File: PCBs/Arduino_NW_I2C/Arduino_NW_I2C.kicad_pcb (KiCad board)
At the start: 2 copper layers, 68.6 x 53.3 mm, 22 parts, among them J1 PT_Conn_01x04, J10 PT_Conn_01x04, J11 PT_Conn_01x04, J12 PT_Conn_01x04, J13 PT_Conn_01x04, J14 Conn_01x02_Female, J2 PT_Conn_01x06, J3 PT_Conn_01x06, J4 PT_Conn_01x06, J5 PT_Conn_01x06, J6 Conn_01x08_Female, J7 Conn_01x08_Female, J8 Conn_01x08_Female, J9 PT_Conn_01x04, U1 PT_Ethernet_Shield, U2 MUX

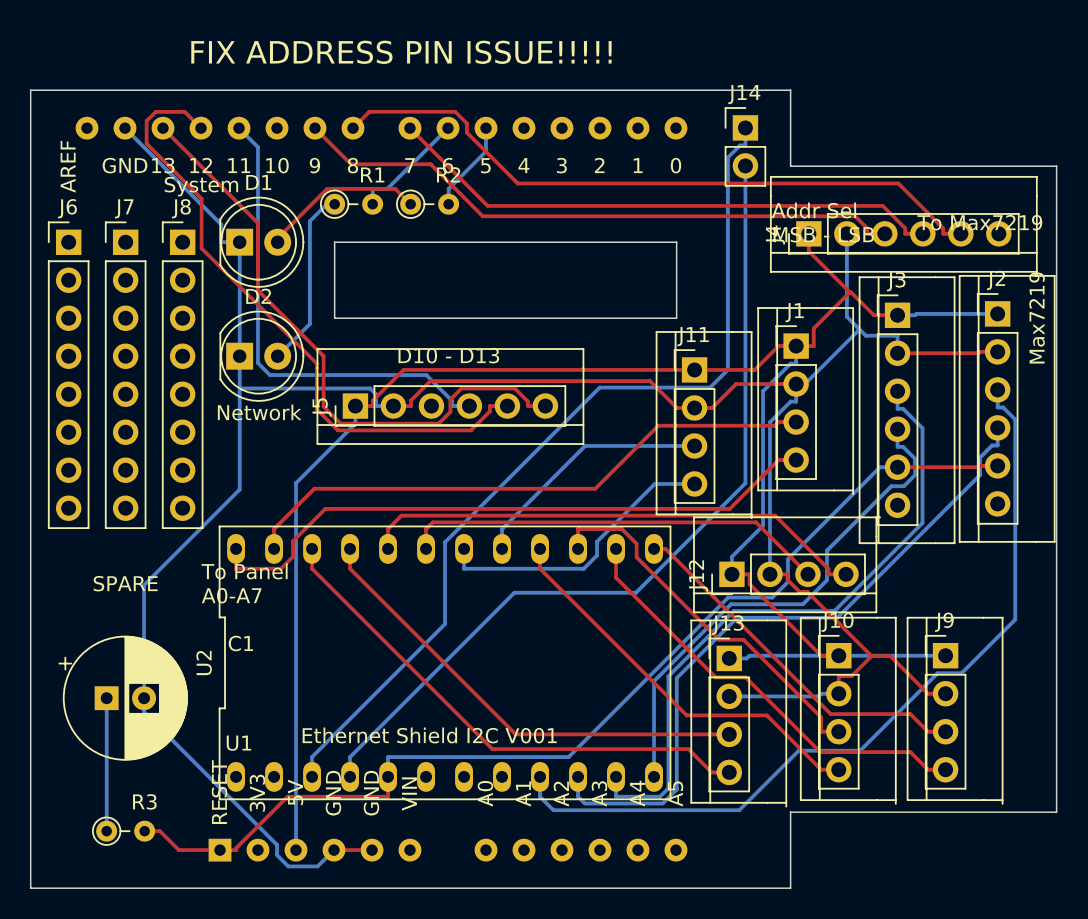
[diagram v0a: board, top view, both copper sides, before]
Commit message: PCB WORK
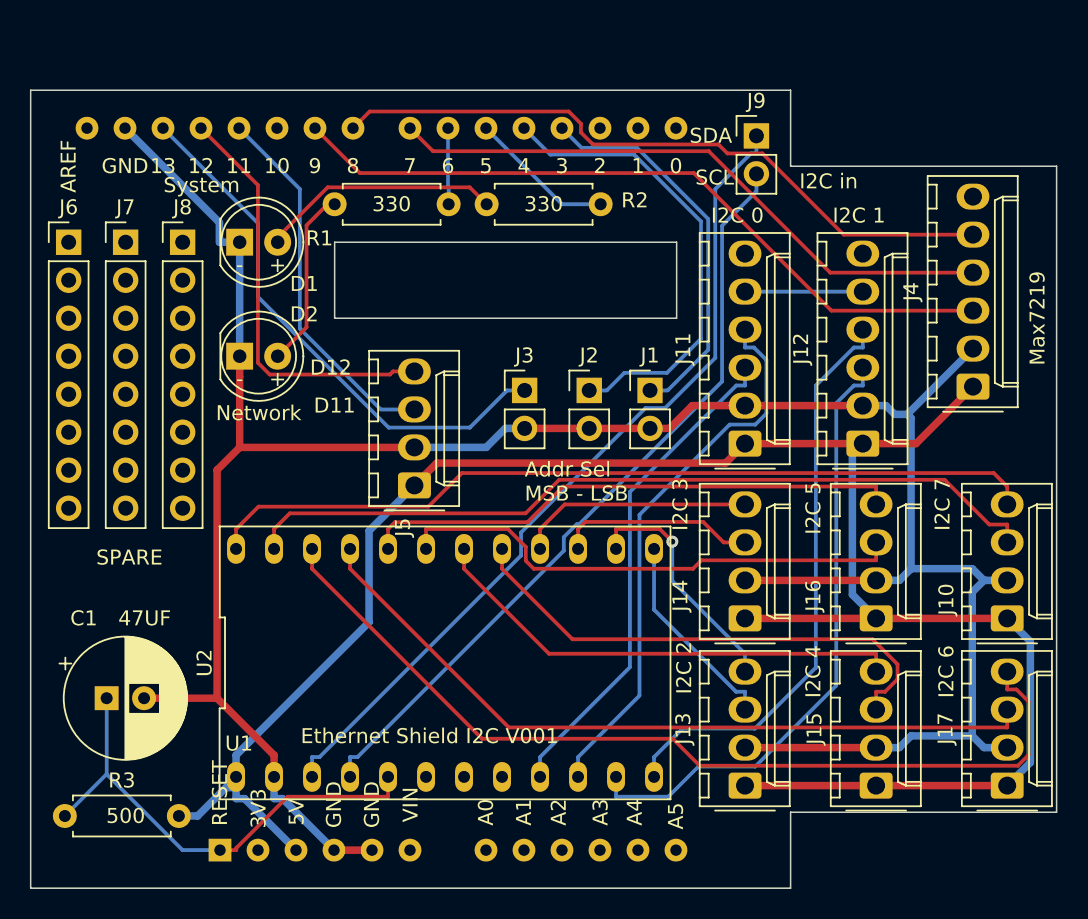
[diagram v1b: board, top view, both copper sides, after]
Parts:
- removed the J10 at (152.4, 101.0)
- added J1: A0, Connector_PinHeader_2.54mm:PinHeader_1x02_P2.54mm_Vertical, F.Cu at (139.8, 83.3)
- added J14: PT_Conn_01x04, PT_Library_v001:Molex_1x04_P2.54mm_Vertical, F.Cu at (146.2, 98.6)
- added J2: A1, Connector_PinHeader_2.54mm:PinHeader_1x02_P2.54mm_Vertical, F.Cu at (135.7, 83.3)
- added J3: A2, Connector_PinHeader_2.54mm:PinHeader_1x02_P2.54mm_Vertical, F.Cu at (131.4, 83.3)
- J10: renamed from J1; footprint PT_Library_v001:PT_PinHeader_1x04_P2.54mm_Vertical -> PT_Library_v001:Molex_1x04_P2.54mm_Vertical
- J11: renamed from J2; footprint PT_Library_v001:PT_PinHeader_1x06_P2.54mm_Vertical -> PT_Library_v001:Molex_1x06_P2.54mm_Vertical
- J12: renamed from J3; footprint PT_Library_v001:PT_PinHeader_1x06_P2.54mm_Vertical -> PT_Library_v001:Molex_1x06_P2.54mm_Vertical
- J13: renamed from J9; footprint PT_Library_v001:PT_PinHeader_1x04_P2.54mm_Vertical -> PT_Library_v001:Molex_1x04_P2.54mm_Vertical
- J15: renamed from J11; footprint PT_Library_v001:PT_PinHeader_1x04_P2.54mm_Vertical -> PT_Library_v001:Molex_1x04_P2.54mm_Vertical
- J16: renamed from J12; footprint PT_Library_v001:PT_PinHeader_1x04_P2.54mm_Vertical -> PT_Library_v001:Molex_1x04_P2.54mm_Vertical
- J17: renamed from J13; footprint PT_Library_v001:PT_PinHeader_1x04_P2.54mm_Vertical -> PT_Library_v001:Molex_1x04_P2.54mm_Vertical
- J4: footprint PT_Library_v001:PT_PinHeader_1x06_P2.54mm_Vertical -> PT_Library_v001:Molex_1x06_P2.54mm_Vertical
- J5: footprint PT_Library_v001:PT_PinHeader_1x06_P2.54mm_Vertical -> PT_Library_v001:Molex_1x04_P2.54mm_Vertical
- R1, R2, R3: footprint PT_Library_v001:PT_R_Axial_DIN0204_L3.6mm_D1.6mm_P2.54mm_Vertical -> PT_Library_v001:R_Axial_DIN0207_L6.3mm_D2.5mm_P7.62mm_Horizontal
- moved J15 30.3 mm to (154.9, 109.7), turned to 90 degrees
- moved J10 23.0 mm to (163.7, 98.6), turned to 90 degrees
- moved J17 20.4 mm to (163.7, 109.7), turned to 90 degrees
- moved J11 19.0 mm to (146.2, 86.9), turned to 90 degrees
- moved J13 16.0 mm to (146.2, 109.7), turned to 90 degrees
- moved J4 15.0 mm to (161.4, 83.1)
- moved J16 10.1 mm to (154.9, 98.6)
- moved J12 8.89 mm to (154.0, 86.9), turned to 90 degrees
- moved J5 6.61 mm to (124.1, 89.7)
- moved R2 5.08 mm to (128.9, 70.9)
- moved R3 2.97 mm to (100.7, 111.8)
- moved J9 0.90 mm to (146.9, 66.3)
- renumbered J14 to J9
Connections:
- R3 pad 2: /RST -> +5V
- U1 pad 1: /RST -> Net-(C1-Pad1)
- U1 pad 24: Net-(J5-Pad4) -> Net-(J5-Pad3)
- U1 pad 25: Net-(J5-Pad5) -> Net-(J5-Pad4)
- U1 pad 26: Net-(J5-Pad6) -> Net-(J3-Pad1)
- U2 pad +5V: Net-(U2-Pad+5V) -> +5V
- U2 pad GND: Net-(U2-PadGND) -> GND
- U2 pad RST: /RST -> Net-(C1-Pad1)
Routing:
- net /RST: track 70.7 -> 7.87 mm
- net Net-(J5-Pad5): track 42.5 -> 0.00 mm
- net Net-(J5-Pad6): track 40.5 -> 0.00 mm
- net Net-(J3-Pad1): track 0.00 -> 36.4 mm
- net Net-(J2-Pad1): track 0.00 -> 31.2 mm
- net /SD6: track 34.9 -> 61.5 mm
- net Net-(J1-Pad1): track 0.00 -> 26.0 mm
- net Net-(J5-Pad3): track 0.00 -> 25.0 mm
- net Net-(C1-Pad1): track 8.89 -> 32.8 mm
- net /SC0: track 54.8 -> 33.4 mm
- net /SC6: track 31.3 -> 50.8 mm
- net /SC4: track 16.5 -> 34.4 mm
- net /SC7: track 39.2 -> 54.1 mm
- net /SD7: track 42.4 -> 56.0 mm
- net /SD2: track 29.3 -> 16.1 mm, vias 0 -> 1
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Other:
- net class POWER added: clearance 0.2, trace_width 0.5, via_dia 0.8, via_drill 0.4
- board text added: "+"
- board text added: "-"
- board text added: "330"
- board text added: "47UF"
- board text added: "500"
- board text added: "D11"
- board text added: "D12"
- board text added: "I2C 0"
- board text added: "I2C 1"
- board text added: "I2C 2"
- board text added: "I2C 3"
- board text added: "I2C 4"
- board text added: "I2C 5"
- board text added: "I2C 6"
- board text added: "I2C 7"
- board text added: "I2C in"
- board text added: "SCL"
- board text added: "SDA"
- board text removed: "D10 - D13"
- board text removed: "FIX ADDRESS PIN ISSUE!!!!!"
- board text removed: "To Max7219"
- board text removed: "To Panel A0-A7"
